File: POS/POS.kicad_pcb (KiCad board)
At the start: 4 copper layers, 30.5 x 17.8 mm, 34 parts, among them J1 uFL, J2 Coax, U1 MPU-9250, U2 AP2112K-1.8, U3 SIM28ML

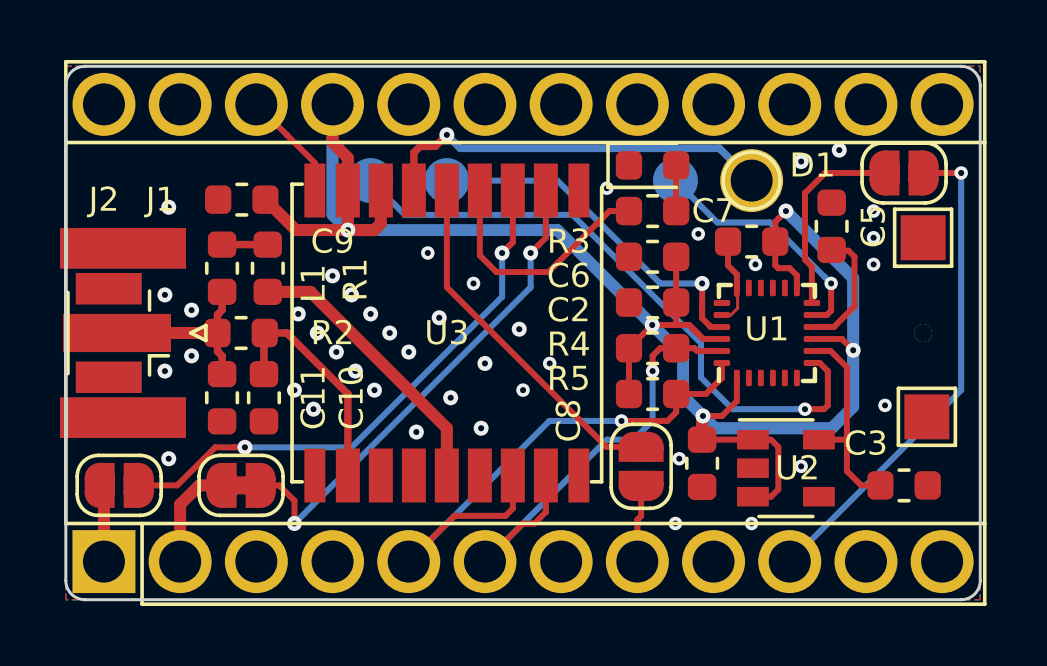
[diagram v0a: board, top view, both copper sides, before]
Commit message: major cleanup and fixes
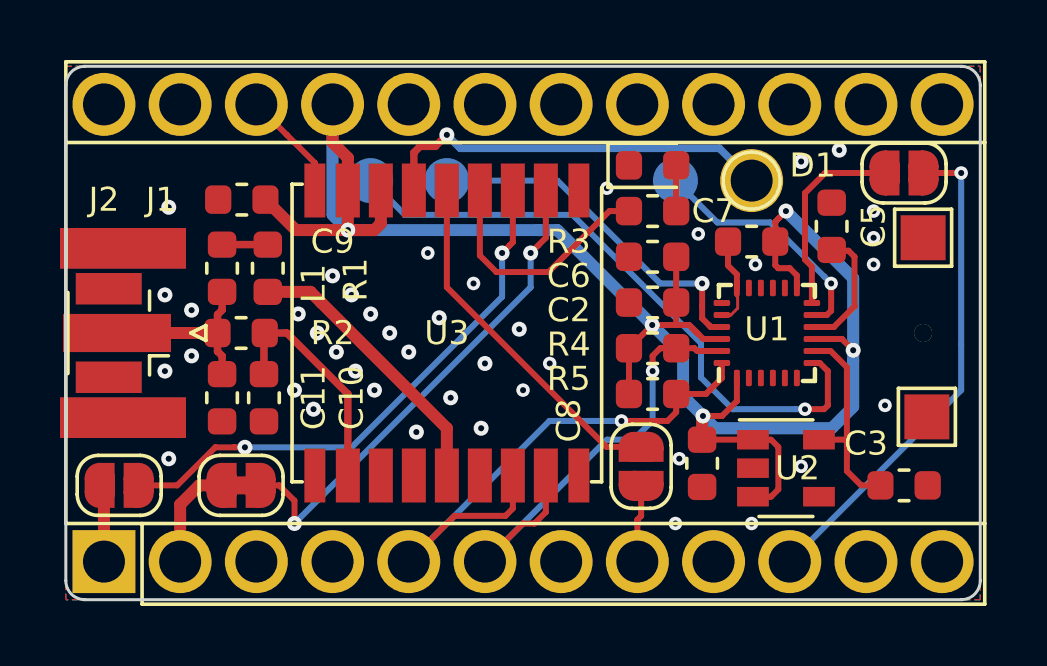
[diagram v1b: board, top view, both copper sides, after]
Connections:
- net ~RST renamed ~{RST}
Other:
- net class Default removed
- net class Power removed
- net class small removed
- net class tiny removed
- board text added: "~{RST}"
- board text removed: "~RST"
